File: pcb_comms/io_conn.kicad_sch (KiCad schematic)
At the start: 23 parts, among them IC1 CP2102N-A02-GQFN28, J1 Conn_01x06_Pin, J2 USB_B_Micro, J3 OBC_I2C, J5 OBC_I2C, J6 OBC_I2C, U6 ADP122AUJZ-3.3-R7

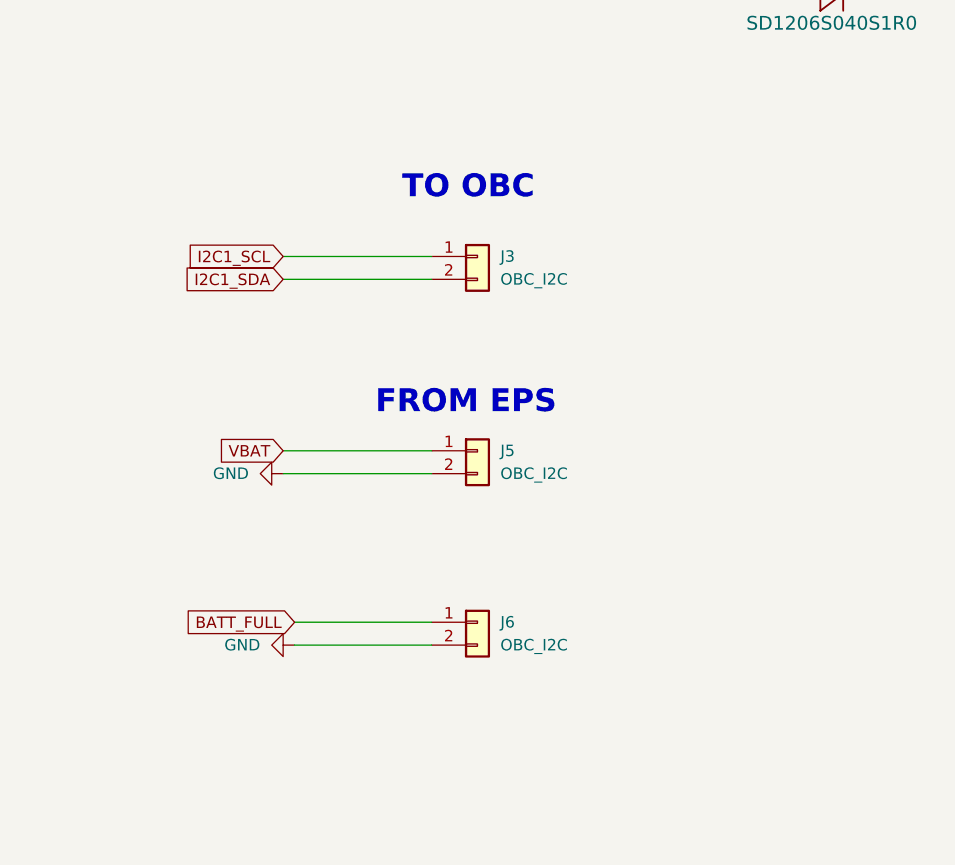
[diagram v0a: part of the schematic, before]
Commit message: rev 1.1
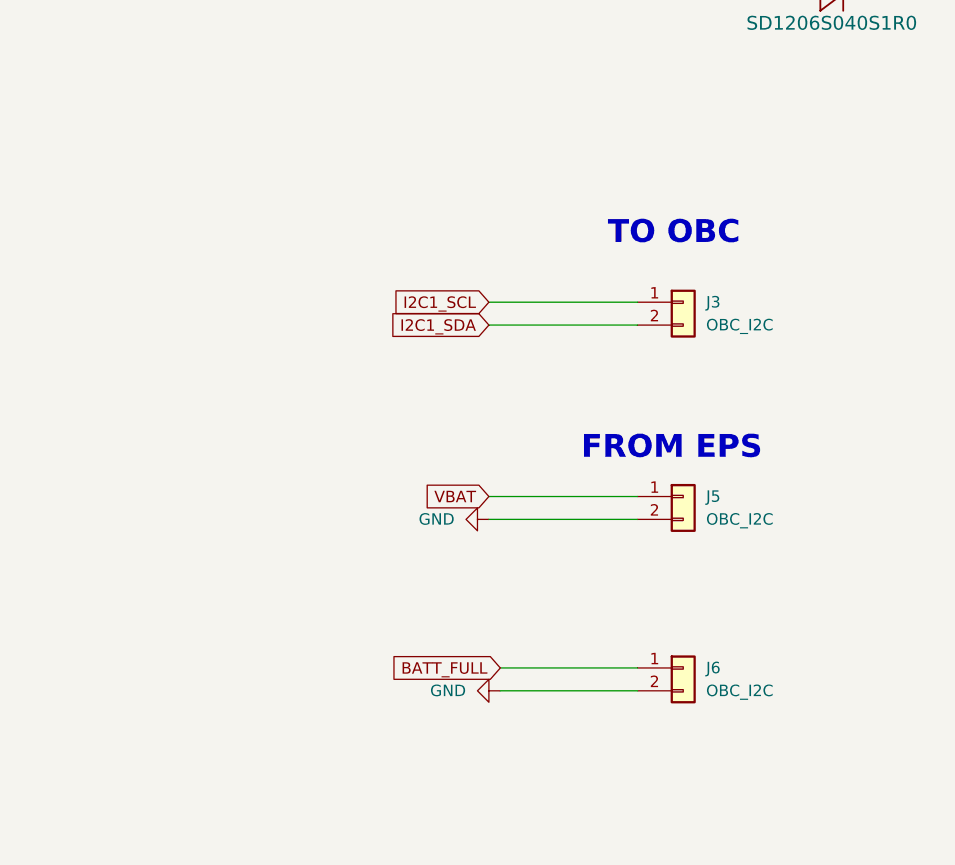
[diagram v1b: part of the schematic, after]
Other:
- moved on the sheet: J3, J5, J6
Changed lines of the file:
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@@
 	(text "TO OBC"
 		(exclude_from_sim no)
-		(at 212.344 63.5 0)
+		(at 235.204 68.58 0)
 		(effects
 			(font
@@
 	(text "FROM EPS"
 		(exclude_from_sim no)
-		(at 212.09 87.376 0)
+		(at 234.95 92.456 0)
 		(effects
 			(font
@@
 	(wire
 		(pts
-			(xy 191.77 92.71) (xy 208.28 92.71)
+			(xy 214.63 97.79) (xy 231.14 97.79)
 		)
 		(stroke
@@
 	(wire
 		(pts
-			(xy 193.04 111.76) (xy 208.28 111.76)
+			(xy 215.9 116.84) (xy 231.14 116.84)
 		)
 		(stroke
@@
 	(wire
 		(pts
-			(xy 191.77 95.25) (xy 208.28 95.25)
+			(xy 214.63 100.33) (xy 231.14 100.33)
 		)
 		(stroke
@@
 	(wire
 		(pts
-			(xy 191.77 71.12) (xy 208.28 71.12)
+			(xy 214.63 76.2) (xy 231.14 76.2)
 		)
 		(stroke
@@
 	(wire
 		(pts
-			(xy 193.04 114.3) (xy 208.28 114.3)
+			(xy 215.9 119.38) (xy 231.14 119.38)
 		)
 		(stroke
@@
 	(wire
 		(pts
-			(xy 191.77 73.66) (xy 208.28 73.66)
+			(xy 214.63 78.74) (xy 231.14 78.74)
 		)
 		(stroke
@@
 	(global_label "VBAT"
 		(shape input)
-		(at 191.77 92.71 180)
+		(at 214.63 97.79 180)
 		(fields_autoplaced yes)
 		(effects
@@
 		)
 		(property "Intersheetrefs" "${INTERSHEET_REFS}"
-			(at 184.37 92.71 0)
+			(at 207.23 97.79 0)
 			(effects
 				(font
@@
 	(global_label "I2C1_SDA"
 		(shape input)
-		(at 191.77 73.66 180)
+		(at 214.63 78.74 180)
 		(fields_autoplaced yes)
 		(effects
@@
 		)
 		(property "Intersheetrefs" "${INTERSHEET_REFS}"
-			(at 179.9553 73.66 0)
+			(at 202.8153 78.74 0)
 			(effects
 				(font
@@
 	(global_label "I2C1_SCL"
 		(shape input)
-		(at 191.77 71.12 180)
+		(at 214.63 76.2 180)
 		(fields_autoplaced yes)
 		(effects
@@
 		)
 		(property "Intersheetrefs" "${INTERSHEET_REFS}"
-			(at 180.0158 71.12 0)
+			(at 202.8758 76.2 0)
 			(effects
 				(font
@@
 	(global_label "BATT_FULL"
 		(shape input)
-		(at 193.04 111.76 180)
+		(at 215.9 116.84 180)
 		(fields_autoplaced yes)
 		(effects
@@
 		)
 		(property "Intersheetrefs" "${INTERSHEET_REFS}"
-			(at 180.3181 111.76 0)
+			(at 203.1781 116.84 0)
 			(effects
 				(font
@@
 	(symbol
 		(lib_id "Connector_Generic:Conn_01x02")
-		(at 213.36 71.12 0)
+		(at 236.22 76.2 0)
 		(unit 1)
 		(exclude_from_sim no)
@@
 		(fields_autoplaced yes)
 		(property "Reference" "J3"
-			(at 215.9 71.1199 0)
+			(at 238.76 76.1999 0)
 			(effects
 				(font
@@
 		)
 		(property "Value" "OBC_I2C"
-			(at 215.9 73.6599 0)
+			(at 238.76 78.7399 0)
 			(effects
 				(font
@@
 		)
 		(property "Footprint" ""
-			(at 213.36 71.12 0)
+			(at 236.22 76.2 0)
 			(effects
 				(font
@@
 		)
 		(property "Datasheet" "~"
-			(at 213.36 71.12 0)
+			(at 236.22 76.2 0)
 			(effects
 				(font
@@
 		)
 		(property "Description" "Generic connector, single row, 01x02, script generated (kicad-library-utils/schlib/autogen/connector/)"
-			(at 213.36 71.12 0)
+			(at 236.22 76.2 0)
 			(effects
 				(font
@@
 	(symbol
 		(lib_id "Connector_Generic:Conn_01x02")
-		(at 213.36 92.71 0)
+		(at 236.22 97.79 0)
 		(unit 1)
 		(exclude_from_sim no)
@@
 		(fields_autoplaced yes)
 		(property "Reference" "J5"
-			(at 215.9 92.7099 0)
+			(at 238.76 97.7899 0)
 			(effects
 				(font
@@
 		)
 		(property "Value" "OBC_I2C"
-			(at 215.9 95.2499 0)
+			(at 238.76 100.3299 0)
 			(effects
 				(font
@@
 		)
 		(property "Footprint" ""
-			(at 213.36 92.71 0)
+			(at 236.22 97.79 0)
 			(effects
 				(font
@@
 		)
 		(property "Datasheet" "~"
-			(at 213.36 92.71 0)
+			(at 236.22 97.79 0)
 			(effects
 				(font
@@
 		)
 		(property "Description" "Generic connector, single row, 01x02, script generated (kicad-library-utils/schlib/autogen/connector/)"
-			(at 213.36 92.71 0)
+			(at 236.22 97.79 0)
 			(effects
 				(font
@@
 	(symbol
 		(lib_id "power:GND")
-		(at 193.04 114.3 270)
+		(at 215.9 119.38 270)
 		(unit 1)
 		(exclude_from_sim no)
@@
 		(fields_autoplaced yes)
 		(property "Reference" "#PWR069"
-			(at 186.69 114.3 0)
+			(at 209.55 119.38 0)
 			(effects
 				(font
@@
 		)
 		(property "Value" "GND"
-			(at 189.23 114.2999 90)
+			(at 212.09 119.3799 90)
 			(effects
 				(font
@@
 		)
 		(property "Footprint" ""
-			(at 193.04 114.3 0)
+			(at 215.9 119.38 0)
 			(effects
 				(font
@@
 		)
 		(property "Datasheet" ""
-			(at 193.04 114.3 0)
+			(at 215.9 119.38 0)
 			(effects
 				(font
@@
 		)
 		(property "Description" "Power symbol creates a global label with name \"GND\" , ground"
-			(at 193.04 114.3 0)
+			(at 215.9 119.38 0)
 			(effects
 				(font
@@
 	(symbol
 		(lib_id "Connector_Generic:Conn_01x02")
-		(at 213.36 111.76 0)
+		(at 236.22 116.84 0)
 		(unit 1)
 		(exclude_from_sim no)
@@
 		(fields_autoplaced yes)
 		(property "Reference" "J6"
-			(at 215.9 111.7599 0)
+			(at 238.76 116.8399 0)
 			(effects
 				(font
@@
 		)
 		(property "Value" "OBC_I2C"
-			(at 215.9 114.2999 0)
+			(at 238.76 119.3799 0)
 			(effects
 				(font
@@
 		)
 		(property "Footprint" ""
-			(at 213.36 111.76 0)
+			(at 236.22 116.84 0)
 			(effects
 				(font
@@
 		)
 		(property "Datasheet" "~"
-			(at 213.36 111.76 0)
+			(at 236.22 116.84 0)
 			(effects
 				(font
@@
 		)
 		(property "Description" "Generic connector, single row, 01x02, script generated (kicad-library-utils/schlib/autogen/connector/)"
-			(at 213.36 111.76 0)
+			(at 236.22 116.84 0)
 			(effects
 				(font
@@
 	(symbol
 		(lib_id "power:GND")
-		(at 191.77 95.25 270)
+		(at 214.63 100.33 270)
 		(unit 1)
 		(exclude_from_sim no)
@@
 		(fields_autoplaced yes)
 		(property "Reference" "#PWR051"
-			(at 185.42 95.25 0)
+			(at 208.28 100.33 0)
 			(effects
 				(font
@@
 		)
 		(property "Value" "GND"
-			(at 187.96 95.2499 90)
+			(at 210.82 100.3299 90)
 			(effects
 				(font
@@
 		)
 		(property "Footprint" ""
-			(at 191.77 95.25 0)
+			(at 214.63 100.33 0)
 			(effects
 				(font
@@
 		)
 		(property "Datasheet" ""
-			(at 191.77 95.25 0)
+			(at 214.63 100.33 0)
 			(effects
 				(font
@@
 		)
 		(property "Description" "Power symbol creates a global label with name \"GND\" , ground"
-			(at 191.77 95.25 0)
+			(at 214.63 100.33 0)
 			(effects
 				(font
